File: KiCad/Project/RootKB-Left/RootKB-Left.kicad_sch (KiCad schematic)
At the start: 70 parts, among them J1 OLED-128x32, SW1 Switch, U1 Arduino_Pro_Micro, U2 TRRS

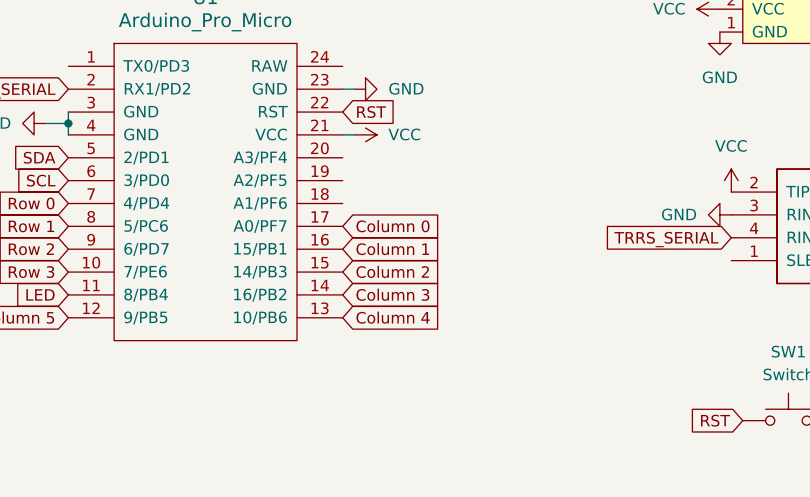
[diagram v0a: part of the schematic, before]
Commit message: routing left
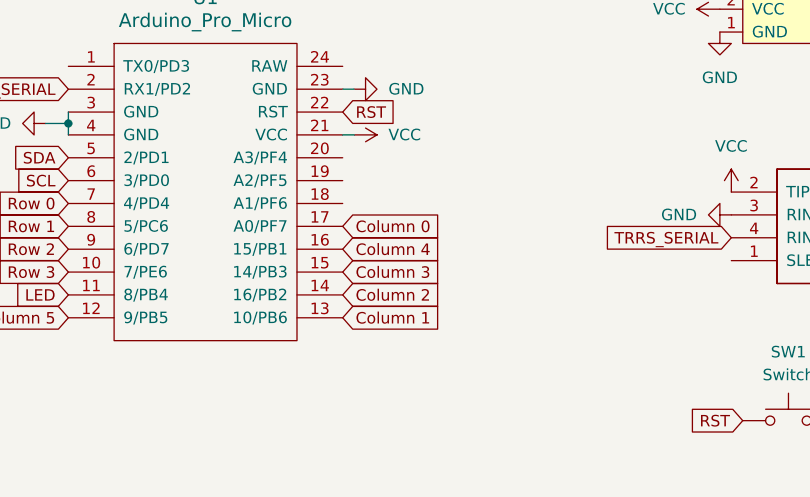
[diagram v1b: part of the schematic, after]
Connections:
- net Column 1: now also U1.13 (10/PB6); no longer U1.16 (15/PB1)
- net Column 2: now also U1.14 (16/PB2); no longer U1.15 (14/PB3)
- net Column 3: now also U1.15 (14/PB3); no longer U1.14 (16/PB2)
- net Column 4: now also U1.16 (15/PB1); no longer U1.13 (10/PB6)
